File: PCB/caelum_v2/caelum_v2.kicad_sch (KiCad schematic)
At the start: 41 parts, among them J1 SS445P, J2 i2C Bus2, J4 Batt, J5 DRV5032DULPG(M), J7 I2C BUS1, J8 DS18B20, Q1 FS8205A-FC, Q2 BSS138, Q3 Si2323DS, U1 DW01A, U2 MCP1825S, U3 ESP32-H2-SUPERMINI, U5 LPS22HB

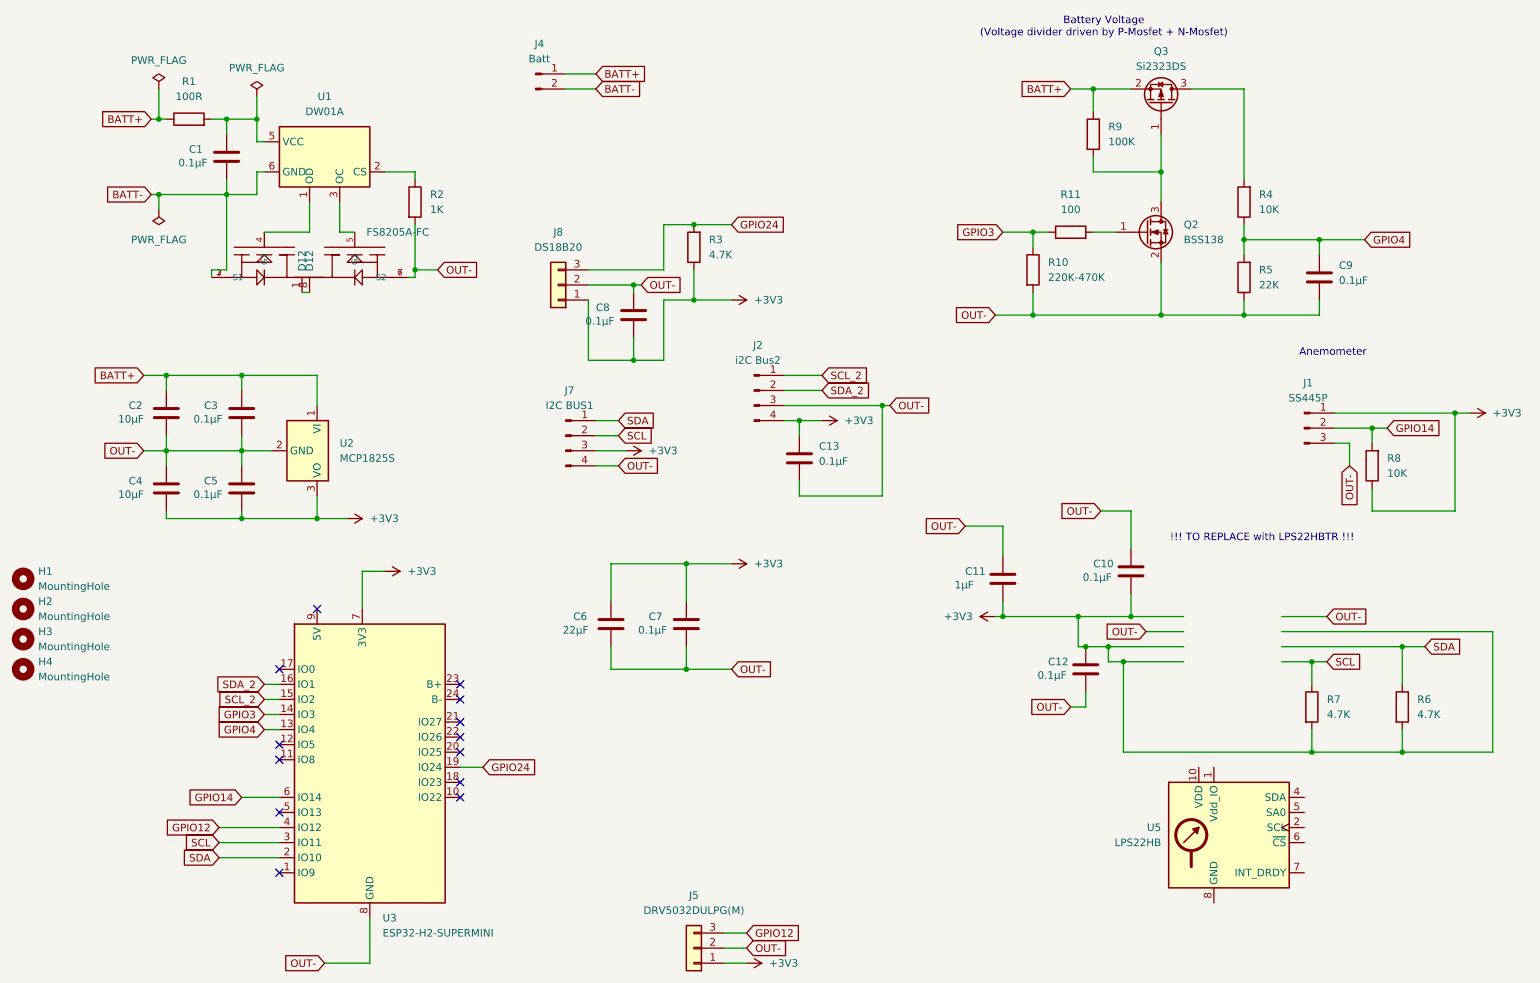
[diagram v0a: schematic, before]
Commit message: Refactor code structure for improved readability and maintainability
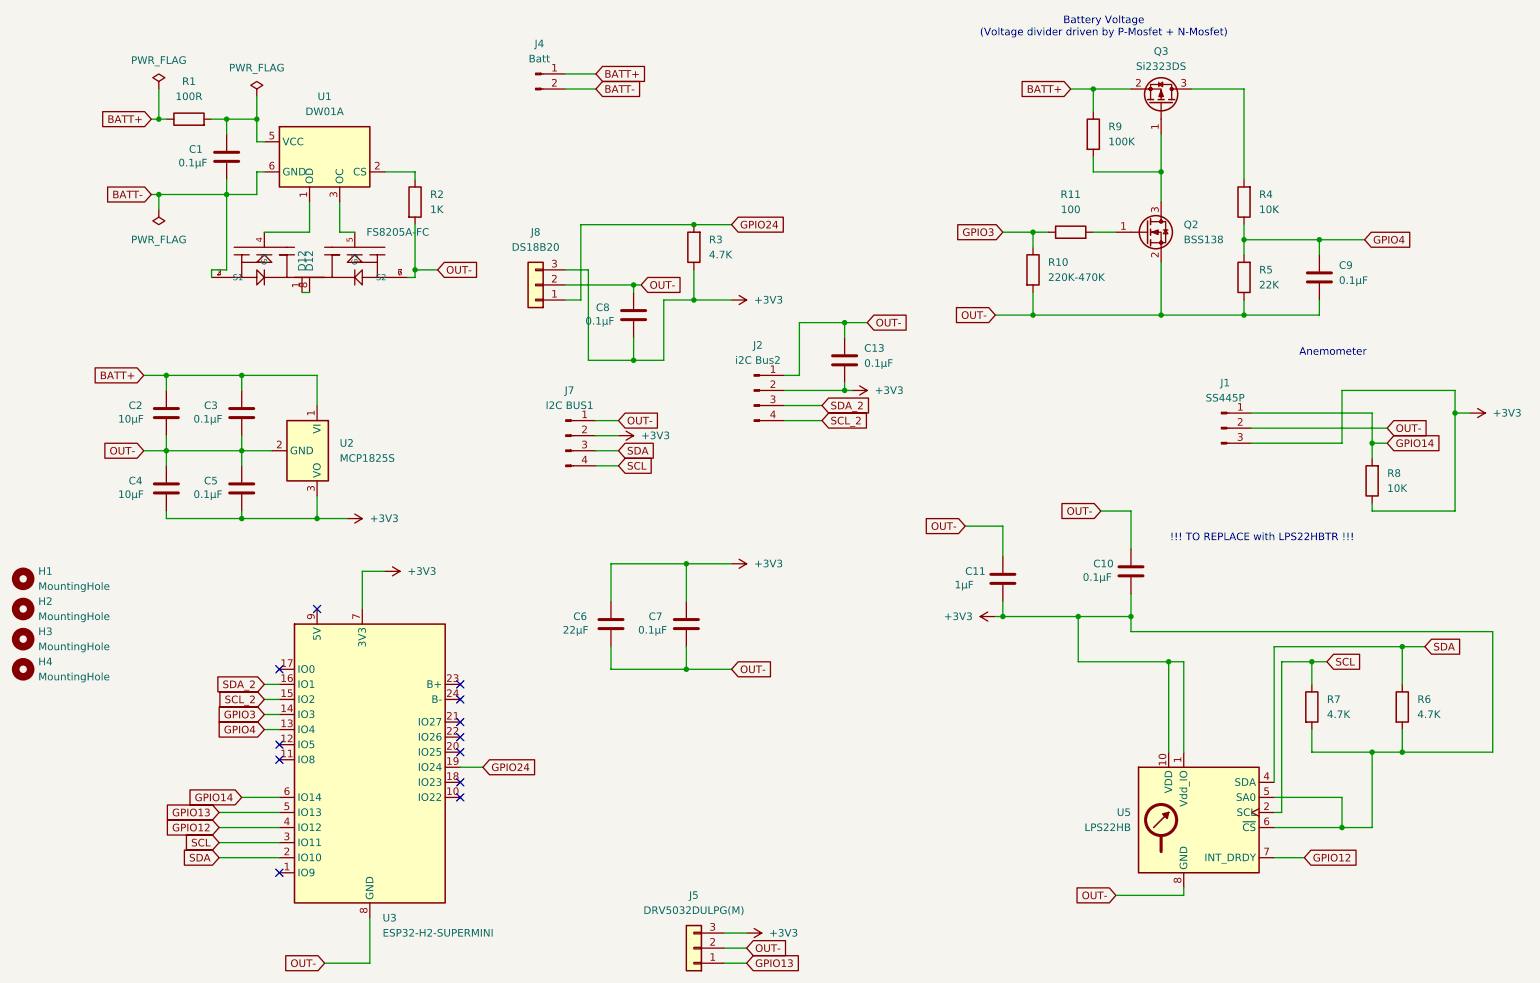
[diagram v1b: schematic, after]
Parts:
- removed C12: 0.1µF, Capacitor_SMD:C_0805_2012Metric, symbol Device:C
- J1, J5, J8: footprint Connector_Hirose:Hirose_DF13C_CL535-0403-5-51_1x03-1MP_P1.25mm_Vertical -> Connector_JST:JST_PH_B3B-PH-SM4-TB_1x03-1MP_P2.00mm_Vertical
- J2: footprint Connector_JST:JST_PH_B4B-PH-SM4-TB_1x04-1MP_P2.00mm_Vertical -> Connector_JST:JST_PH_S4B-PH-SM4-TB_1x04-1MP_P2.00mm_Horizontal
- J4: footprint Connector_PinHeader_2.54mm:PinHeader_1x02_P2.54mm_Vertical -> Connector_JST:JST_PH_S2B-PH-SM4-TB_1x02-1MP_P2.00mm_Horizontal
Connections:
- net +3V3: now also C13.2, J1.3 (Pin_3), J2.2 (Pin_2), J5.3 (Pin_3), J7.2 (Pin_2), J8.3 (Pin_3), U5.1 (Vdd_IO), U5.10 (VDD), U5.5 (SA0), U5.6 (~{CS}); no longer C13.1, J1.1 (Pin_1), J2.4 (Pin_4), J5.1 (Pin_1), J7.3 (Pin_3), J8.1 (Pin_1)
- net GPIO12: now also U5.7 (INT_DRDY); no longer J5.3 (Pin_3)
- net GPIO14: now also J1.1 (Pin_1); no longer J1.2 (Pin_2)
- net GPIO24: now also J8.1 (Pin_1); no longer J8.3 (Pin_3)
- net OUT-: now also C13.1, J1.2 (Pin_2), J2.1 (Pin_1), J7.1 (Pin_1), U5.3 (GND), U5.8 (GND), U5.9 (GND); no longer C13.2, J1.3 (Pin_3), J2.3 (Pin_3), J7.4 (Pin_4)
- net SCL: now also J7.4 (Pin_4), U5.2 (SCL); no longer J7.2 (Pin_2)
- net SCL_2: now also J2.4 (Pin_4); no longer J2.1 (Pin_1)
- net SDA: now also J7.3 (Pin_3), U5.4 (SDA); no longer J7.1 (Pin_1)
- net SDA_2: now also J2.3 (Pin_3); no longer J2.2 (Pin_2)
- net GPIO13: now reaches U3.5 (IO13)
- net GPIO13: now also J5.1 (Pin_1)
- no-connect marks 13 -> 12
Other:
- moved on the sheet: C13, J1, J8, R8, U5
